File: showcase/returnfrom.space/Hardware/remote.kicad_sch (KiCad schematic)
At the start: 4 parts, among them J6 OLED, U12 TP4056, U2 ESP32-S2-MINI-1

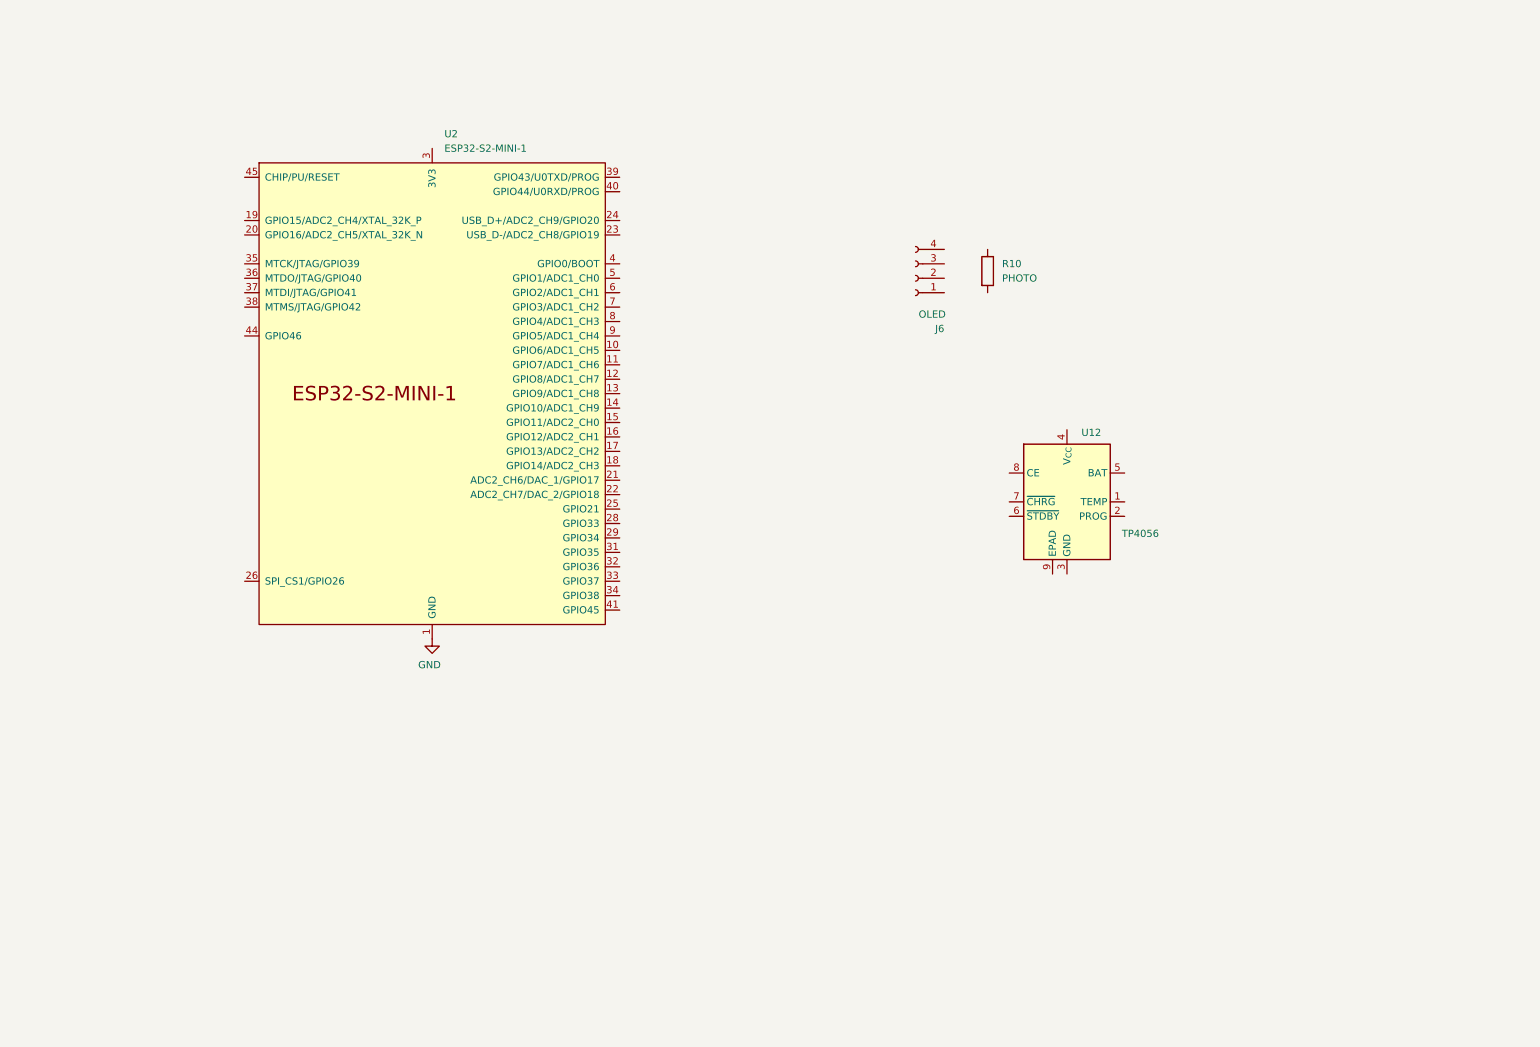
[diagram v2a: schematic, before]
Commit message: board almost done
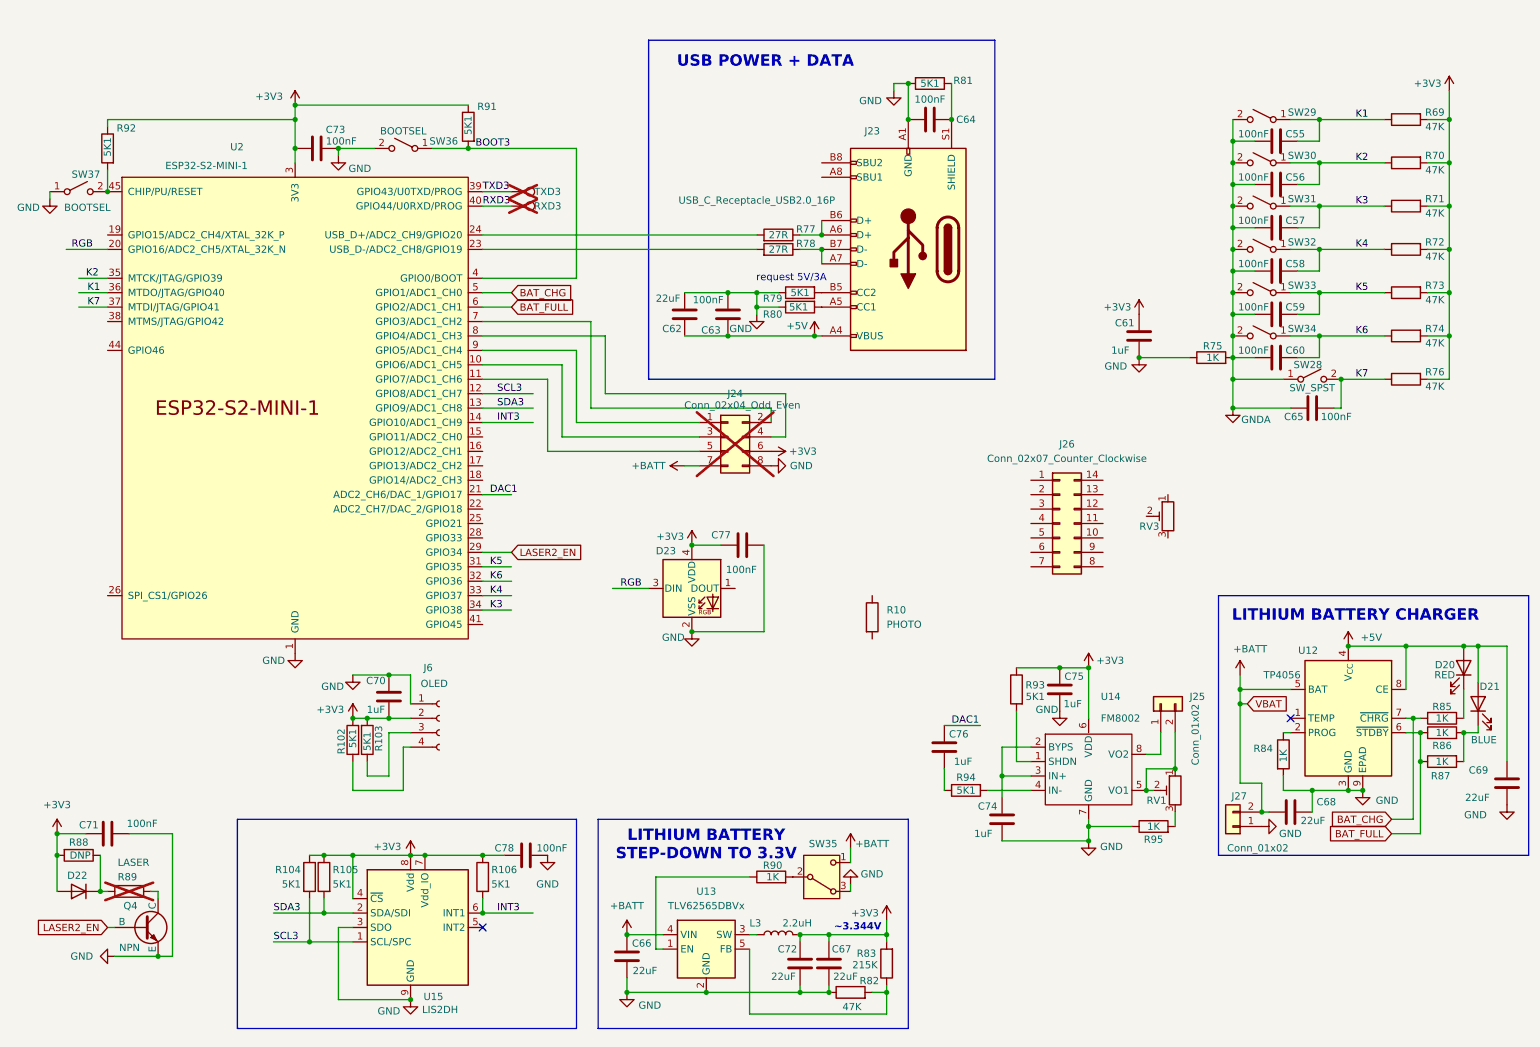
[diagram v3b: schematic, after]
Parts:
- added C55, C56, C57, C58, C59, C60, C63, C64, C65, C71, C73, C77, C78: 100nF, Capacitor_SMD:C_0402_1005Metric, symbol Device:C
- added C61, C70, C74, C75, C76: 1uF, Capacitor_SMD:C_0402_1005Metric, symbol Device:C
- added C62, C66, C67, C68, C69, C72: 22uF, Capacitor_SMD:C_0805_2012Metric, symbol Device:C
- added D20: RED, LED_SMD:LED_0603_1608Metric, symbol Device:LED
- added D21: BLUE, LED_SMD:LED_0603_1608Metric, symbol Device:LED
- added D22: D, Diode_SMD:D_SOD-323, symbol Device:D
- added D23: WS2812B-2020, LED_SMD:LED_WS2812B-2020_PLCC4_2.0x2.0mm, symbol LED:WS2812B-2020
- added J23: USB_C_Receptacle_USB2.0_16P, Connector_USB:USB_C_Receptacle_HCTL_HC-TYPE-C-16P-01A, symbol Connector:USB_C_Receptacle_USB2.0_16P
- added J24: Conn_02x04_Odd_Even, Connector_PinSocket_2.54mm:PinSocket_2x04_P2.54mm_Vertical, symbol Connector_Generic:Conn_02x04_Odd_Even
- added J25, J27: Conn_01x02, Connector_Hirose:Hirose_DF13-02P-1.25DS_1x02_P1.25mm_Horizontal, symbol Connector_Generic:Conn_01x02
- added J26: Conn_02x07_Counter_Clockwise, Package_DIP:DIP-14_W7.62mm, symbol Connector_Generic:Conn_02x07_Counter_Clockwise
- added L3: 2.2uH, Inductor_SMD:L_Cenker_CKCS201610, symbol Device:L
- added Q4: NPN, Package_TO_SOT_SMD:SOT-23, symbol Simulation_SPICE:NPN
- added R102, R103, R104, R105, R106, R79, R80, R81, R91, R92, R93, R94: 5K1, Resistor_SMD:R_0402_1005Metric, symbol Device:R
- added R69, R70, R71, R72, R73, R74, R76, R82: 47K, Resistor_SMD:R_0402_1005Metric, symbol Device:R
- added R75, R84, R85, R86, R87, R90, R95: 1K, Resistor_SMD:R_0402_1005Metric, symbol Device:R
- added R77, R78: 27R, Resistor_SMD:R_0402_1005Metric, symbol Device:R
- added R83: 215K, Resistor_SMD:R_0402_1005Metric, symbol Device:R
- added R88: DNP, Resistor_SMD:R_0603_1608Metric, symbol Device:R
- added R89: LASER, Resistor_SMD:R_1210_3225Metric, symbol Device:R
- added RV1, RV3: R_Potentiometer_Trim, Potentiometer_THT:Potentiometer_Runtron_RM-065_Vertical, symbol Device:R_Potentiometer_Trim
- added RXD3, TXD3: TestPoint, TestPoint:TestPoint_Pad_D2.0mm, symbol Connector:TestPoint
- added SW28: SW_SPST, Button_Switch_THT:SW_PUSH-12mm, symbol Switch:SW_SPST
- added SW29, SW30, SW31, SW32, SW33, SW34: SW_SPST, Button_Switch_SMD:SW_SPST_TL3305C, symbol Switch:SW_SPST
- added SW35: SW_SPDT_321, Button_Switch_THT:SW_Slide_SPDT_Angled_CK_OS102011MA1Q, symbol Switch:SW_SPDT_321
- added SW36, SW37: BOOTSEL, Button_Switch_SMD:SW_SPST_TL3305C, symbol Switch:SW_SPST
- added U13: TLV62565DBVx, Package_TO_SOT_SMD:SOT-23-5, symbol Regulator_Switching:TLV62565DBVx
- added U14: FM8002, Package_SO:SOIC-8_3.9x4.9mm_P1.27mm, symbol spacescape:FM8002A
- added U15: LIS2DH, Package_LGA:LGA-14_2x2mm_P0.35mm_LayoutBorder3x4y, symbol Sensor_Motion:LIS2DH
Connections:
- net GND: now also J6.1 (Pin_1), U12.3 (GND), U12.9 (EPAD), C61.1, C62.2, C63.2, C64.2, C66.2, C67.2, C68.2, C69.2, C70.1, C71.2, C72.2, C73.1, C74.1, C75.1, C77.2, C78.2, D23.2 (VSS), J23.A1 (GND), J23.A12 (GND), J23.B1 (GND), J23.B12 (GND), J24.8 (Pin_8), J27.1 (Pin_1), Q4.3 (E), R75.1, R79.1, R80.1, R81.2, R82.1, R84.2, R95.1, SW35.3 (A), SW36.2 (B), SW37.1 (A), U13.2 (GND), U14.7 (GND), U15.10 (GND), U15.11 (GND), U15.12 (GND), U15.13 (GND), U15.14 (GND), U15.3 (SDO), U15.9 (GND)
- net +3V3: now reaches J6.2 (Pin_2)
- net +3V3: now also U2.3 (3V3), C61.2, C67.1, C70.2, C71.1, C72.1, C73.2, C75.2, C77.1, C78.1, D22.2 (A), D23.4 (VDD), J24.6 (Pin_6), L3.2, R102.1, R103.2, R104.1, R105.1, R106.1, R69.2, R70.2, R71.2, R72.2, R73.2, R74.2, R76.2, R83.2, R88.2, R91.1, R92.1, R93.1, U14.6 (VDD), U15.4 (~{CS}), U15.7 (Vdd_IO), U15.8 (Vdd)
- net at J6.3 (Pin_3): now also R103.1
- net at J6.4 (Pin_4): now also R102.2
- net at U12.2 (PROG): now also R84.1
- net +5V: now reaches U12.4 (V_{CC})
- net +5V: now also U12.8 (CE), C62.1, C63.1, C69.1, D20.2 (A), D21.2 (A), J23.A4 (VBUS), J23.A9 (VBUS), J23.B4 (VBUS), J23.B9 (VBUS)
- net +BATT: now reaches U12.5 (BAT)
- net +BATT: now also C66.1, C68.1, J24.7 (Pin_7), J27.2 (Pin_2), SW35.1 (C), U13.4 (VIN)
- net BAT_FULL: now reaches U12.6 (~{STDBY})
- net BAT_FULL: now also U2.6 (GPIO2/ADC1_CH1), R86.1, R87.1
- net BAT_CHG: now reaches U12.7 (~{CHRG})
- net BAT_CHG: now also U2.5 (GPIO1/ADC1_CH0), R85.2
- net at U2.10 (GPIO6/ADC1_CH5): now also J24.3 (Pin_3)
- net at U2.11 (GPIO7/ADC1_CH6): now also J24.5 (Pin_5)
- net SCL3: now reaches U2.12 (GPIO8/ADC1_CH7)
- net SCL3: now also R104.2, U15.1 (SCL/SPC)
- net SDA3: now reaches U2.13 (GPIO9/ADC1_CH8)
- net SDA3: now also R105.2, U15.2 (SDA/SDI)
- net INT3: now reaches U2.14 (GPIO10/ADC1_CH9)
- net INT3: now also R106.2, U15.6 (INT1)
- net RGB: now reaches U2.20 (GPIO16/ADC2_CH5/XTAL_32K_N)
- net RGB: now also D23.3 (DIN)
- net DAC1: now reaches U2.21 (ADC2_CH6/DAC_1/GPIO17)
- net DAC1: now also C76.2
- net at U2.23 (USB_D-/ADC2_CH8/GPIO19): now also R78.2
- net at U2.24 (USB_D+/ADC2_CH9/GPIO20): now also R77.2
- net LASER2_EN: now reaches U2.29 (GPIO34)
- net LASER2_EN: now also Q4.2 (B)
- net K5: now reaches U2.31 (GPIO35)
- net K5: now also C59.2, R73.1, SW33.1 (A)
- net K6: now reaches U2.32 (GPIO36)
- net K6: now also C60.2, R74.1, SW34.1 (A)
- net K4: now reaches U2.33 (GPIO37)
- net K4: now also C58.2, R72.1, SW32.1 (A)
- net K3: now reaches U2.34 (GPIO38)
- net K3: now also C57.2, R71.1, SW31.1 (A)
- net K2: now reaches U2.35 (MTCK/JTAG/GPIO39)
- net K2: now also C56.2, R70.1, SW30.1 (A)
- net K1: now reaches U2.36 (MTDO/JTAG/GPIO40)
- net K1: now also C55.2, R69.1, SW29.1 (A)
- net K7: now reaches U2.37 (MTDI/JTAG/GPIO41)
- net K7: now also C65.2, R76.1, SW28.2 (B)
- net TXD3: now reaches U2.39 (GPIO43/U0TXD/PROG)
- net TXD3: now also TXD3.1
- net BOOT3: now reaches U2.4 (GPIO0/BOOT)
- net BOOT3: now also R91.2, SW36.1 (A)
- net RXD3: now reaches U2.40 (GPIO44/U0RXD/PROG)
- net RXD3: now also RXD3.1
- net at U2.45 (CHIP/PU/RESET): now also R92.2, SW37.2 (B)
- net at U2.7 (GPIO3/ADC1_CH2): now also J24.2 (Pin_2)
- net at U2.8 (GPIO4/ADC1_CH3): now also J24.4 (Pin_4)
- net at U2.9 (GPIO5/ADC1_CH4): now also J24.1 (Pin_1)
- new net: C64.1, J23.S1 (SHIELD), R81.1
- new net: R90.1, U13.1 (EN)
- new net: R90.2, SW35.2 (B)
- new net: R95.2, RV1.3
- new net: D21.1 (K), R86.2, R87.2
- new net: D20.1 (K), R85.1
- new net: R82.2, R83.1, U13.5 (FB)
- new net: R93.2, U14.1 (SHDN)
- new net: J23.B5 (CC2), R79.2
- new net: J25.1 (Pin_1), U14.8 (VO2)
- new net: J25.2 (Pin_2), RV1.1, RV1.2, U14.5 (VO1)
- new net: J23.A5 (CC1), R80.2
- new net: J23.A6 (D+), J23.B6 (D+), R77.1
- new net: J23.A7 (D-), J23.B7 (D-), R78.1
- new net: C74.2, U14.2 (BYPS), U14.3 (IN+)
- new net: Q4.1 (C), R89.1
- new net: D22.1 (K), R88.1, R89.2
- new net: C76.1, R94.1
- new net: R94.2, U14.4 (IN-)
- new net: L3.1, U13.3 (SW)
- new net GNDA: C55.1, C56.1, C57.1, C58.1, C59.1, C60.1, C65.1, R75.2, SW28.1 (A), SW29.2 (B), SW30.2 (B), SW31.2 (B), SW32.2 (B), SW33.2 (B), SW34.2 (B)
- no-connect marks 0 -> 2
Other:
- note added: "LITHIUM BATTERY CHARGER"
- note added: "LITHIUM BATTERY STEP-DOWN TO 3.3V"
- note added: "USB POWER + DATA"
- note added: "request 5V/3A"
- note added: "~3.344V"
- moved on the sheet: J6, R10, U2

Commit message: panelizing...
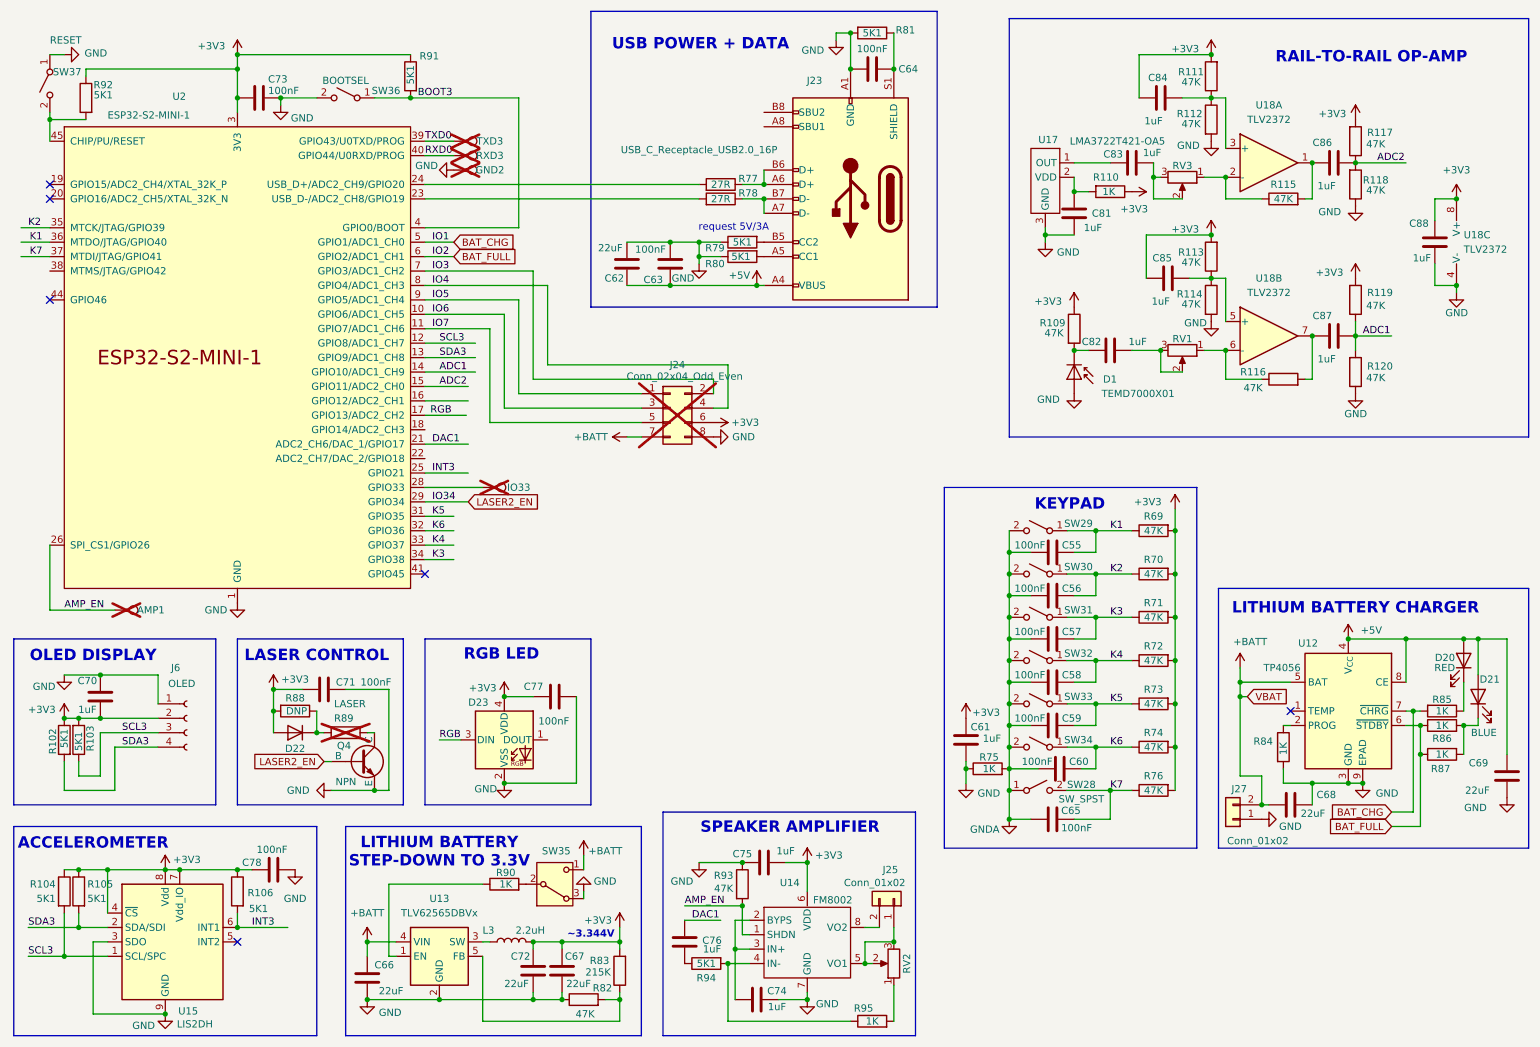
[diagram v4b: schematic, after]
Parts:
- removed J26: Conn_02x07_Counter_Clockwise, Package_DIP:DIP-14_W7.62mm, symbol Connector_Generic:Conn_02x07_Counter_Clockwise
- removed R10: PHOTO, Resistor_SMD:R_1210_3225Metric, symbol Device:R
- removed RV1, RV3: R_Potentiometer_Trim, Potentiometer_THT:Potentiometer_Runtron_RM-065_Vertical, symbol Device:R_Potentiometer_Trim
- added AMP1, GND2, IO33: TestPoint, TestPoint:TestPoint_Pad_D2.0mm, symbol Connector:TestPoint
- added C81, C82, C83, C84, C85, C86, C87, C88: 1uF, Capacitor_SMD:C_0402_1005Metric, symbol Device:C
- added D1: TEMD7000X01, Diode_SMD:D_0805_2012Metric, symbol Sensor_Optical:BPW34-SMD
- added R109, R111, R112, R113, R114, R115, R116, R117, R118, R119, R120: 47K, Resistor_SMD:R_0402_1005Metric, symbol Device:R
- added R110: 1K, Resistor_SMD:R_0402_1005Metric, symbol Device:R
- added RV1, RV2, RV3: R_Potentiometer, Potentiometer_THT:Potentiometer_Runtron_RM-065_Vertical, symbol Device:R_Potentiometer
- added U17: LMA3722T421-OA5, spacescape:LMA3722T421, symbol spacescape:LMA3722T421
- added U18: TLV2372, Package_SO:SOIC-8_3.9x4.9mm_P1.27mm, symbol Amplifier_Operational:TLV2372
- R93: value 5K1 -> 47K
- SW37: value BOOTSEL -> RESET
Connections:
- net +3V3: now also C84.1, C85.1, C88.2, R109.1, R110.1, R111.2, R113.2, R117.2, R119.2, U18.8 (V+); no longer R93.1
- net GND: now also C74.2, R93.1, C81.1, C88.1, D1.2 (A), GND2.1, R112.2, R114.2, R118.1, R120.1, U17.3 (GND), U17.4 (GND), U18.4 (V-); no longer C74.1, R95.1
- net INT3: now also U2.25 (GPIO21); no longer U2.14 (GPIO10/ADC1_CH9)
- net RGB: now also U2.17 (GPIO13/ADC2_CH2); no longer U2.20 (GPIO16/ADC2_CH5/XTAL_32K_N)
- net SCL3: now also J6.3 (Pin_3), R103.1
- net SDA3: now also J6.4 (Pin_4), R102.2
- net at R95.2: now also RV2.1
- net AMP_EN: now reaches R93.2, U14.1 (SHDN)
- net AMP_EN: now also U2.26 (SPI_CS1/GPIO26), AMP1.1
- net at J25.1 (Pin_1): now also U14.5 (VO1), RV2.2, RV2.3; no longer U14.8 (VO2)
- net at J25.2 (Pin_2): now also U14.8 (VO2); no longer U14.5 (VO1)
- net at U14.2 (BYPS), U14.3 (IN+): now also C74.1; no longer C74.2
- net at R94.2, U14.4 (IN-): now also R95.1
- net IO6: now reaches J24.3 (Pin_3), U2.10 (GPIO6/ADC1_CH5)
- net IO7: now reaches J24.5 (Pin_5), U2.11 (GPIO7/ADC1_CH6)
- net ADC2: now reaches U2.15 (GPIO11/ADC2_CH0)
- net ADC2: now also C86.2, R117.1, R118.2
- net at U2.28 (GPIO33): now also IO33.1
- net IO3: now reaches J24.2 (Pin_2), U2.7 (GPIO3/ADC1_CH2)
- net IO4: now reaches J24.4 (Pin_4), U2.8 (GPIO4/ADC1_CH3)
- net IO5: now reaches J24.1 (Pin_1), U2.9 (GPIO5/ADC1_CH4)
- net RXD3 renamed RXD0
- net TXD3 renamed TXD0
- new net: C84.2, R111.1, R112.1, U18.3 (+)
- new net: C85.2, R113.1, R114.1, U18.5 (+)
- new net: C83.1, U17.1 (OUT)
- new net: C81.2, R110.2, U17.2 (VDD)
- new net: R115.1, RV3.1, U18.2 (-)
- new net: C86.1, R115.2, U18.1
- new net: C82.1, D1.1 (K), R109.2
- new net: C82.2, RV1.2, RV1.3
- new net: R116.1, RV1.1, U18.6 (-)
- new net: C87.1, R116.2, U18.7
- new net: C83.2, RV3.2, RV3.3
- new net ADC1: C87.2, R119.1, R120.2, U2.14 (GPIO10/ADC1_CH9)
- no-connect marks 2 -> 6
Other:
- note added: "ACCELEROMETER"
- note added: "KEYPAD"
- note added: "LASER CONTROL"
- note added: "OLED DISPLAY"
- note added: "RAIL-TO-RAIL OP-AMP"
- note added: "RGB LED"
- note added: "SPEAKER AMPLIFIER"
- moved on the sheet: C55, C56, C57, C58, C59, C60, C61, C62, C63, C64, C65, C66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
